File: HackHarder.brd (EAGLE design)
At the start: 30 x 85.3 mm, 8 parts, among them U1 RFM69HW

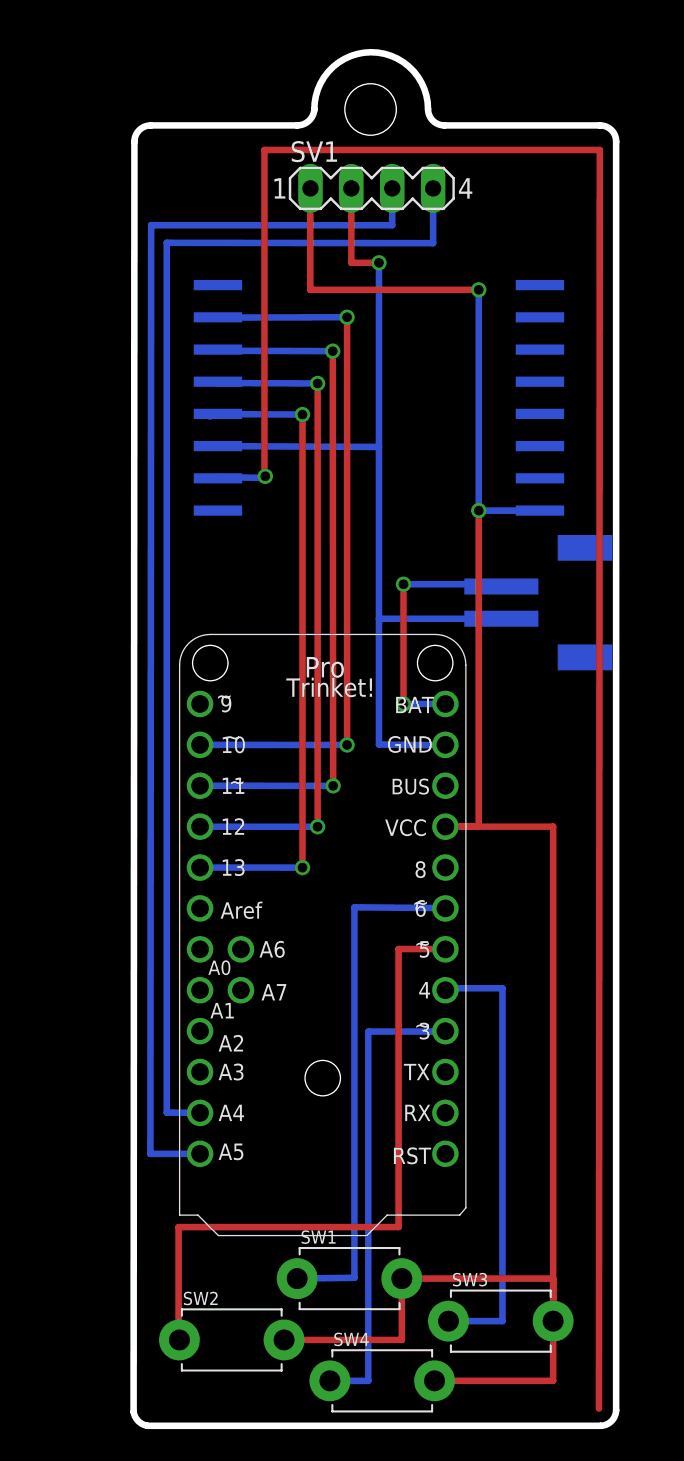
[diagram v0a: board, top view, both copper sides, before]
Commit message: Add files via upload
Latest version
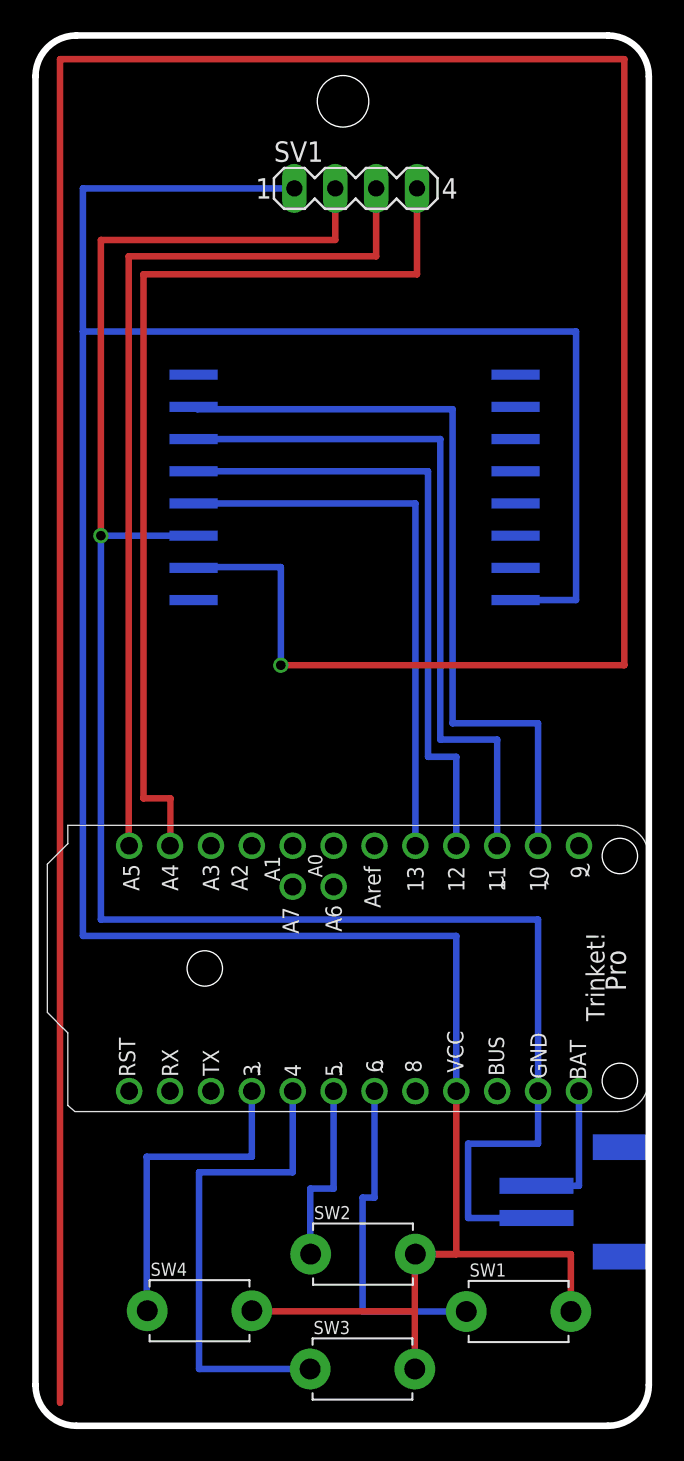
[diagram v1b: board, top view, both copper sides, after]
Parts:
- moved CN1 37.3 mm to (39.9, 11.4)
- moved SW4 12.2 mm to (15.3, 4.61)
- moved SW1 10.7 mm to (35.1, 4.56)
- moved MCU1 10.0 mm to (15.6, 25.9), turned to 270 degrees
- moved SW2 9.74 mm to (25.4, 8.12)
- moved SW3 9.09 mm to (25.4, 0.99)
- moved U1 5.76 mm to (24.9, 54.8)
- moved SV1 1.00 mm to (25.0, 74.3)
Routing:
- net N$11: track 0.00 -> 188.9 mm
- net N$9: track 122.3 -> 0.00 mm
- net G$1: track 58.0 -> 120.0 mm
- net VCC: track 127.7 -> 186.7 mm, vias 2 -> 0
- net N$13: track 40.9 -> 11.6 mm
- net N$3: track 78.0 -> 56.2 mm
- net N$4: track 76.0 -> 59.5 mm
- net N$12: track 32.2 -> 20.9 mm
- net N$15: track 28.9 -> 20.2 mm
- net N$2: track 16.3 -> 8.52 mm, vias 2 -> 0
- net N$8: track 43.7 -> 48.7 mm, vias 2 -> 0
- net N$7: track 39.9 -> 35.0 mm, vias 2 -> 0
- net N$14: track 27.7 -> 30.0 mm
- net N$5: track 42.5 -> 44.1 mm, vias 2 -> 0
- net N$6: track 41.1 -> 39.6 mm, vias 2 -> 0
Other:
- board size 30 x 85.3 mm -> 38.1 x 86.4 mm
